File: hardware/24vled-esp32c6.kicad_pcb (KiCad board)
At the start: 2 copper layers, 26.4 x 90.8 mm, 20 parts, among them J1 2601-1106, J3 Barrel_Jack, Q1 AO3400A, Q2 AO3400A, Q3 AO3400A, Q4 AO3400A, Q5 AO3400A, U1 R-78E5.0-1.0

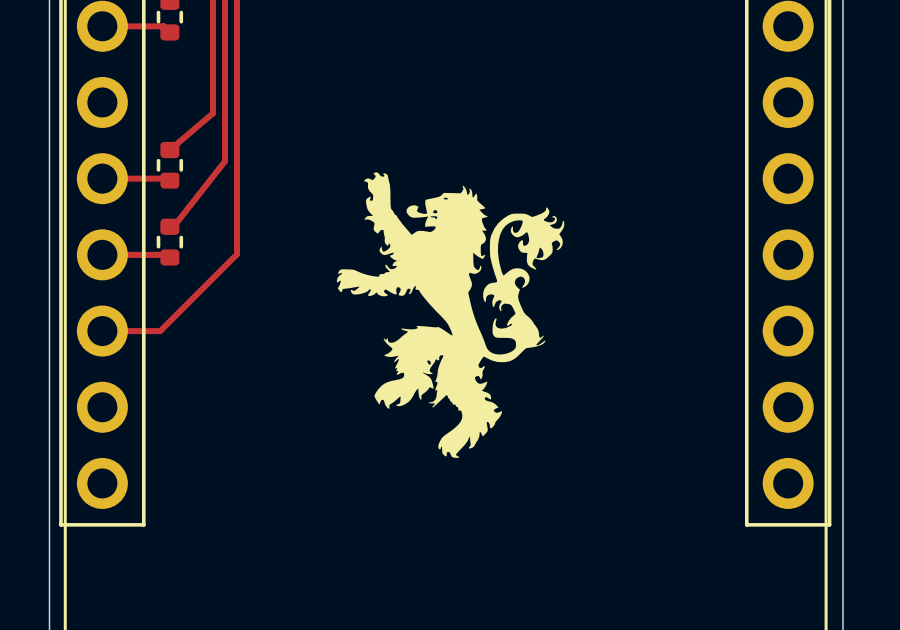
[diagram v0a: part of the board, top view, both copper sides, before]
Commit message: update pages
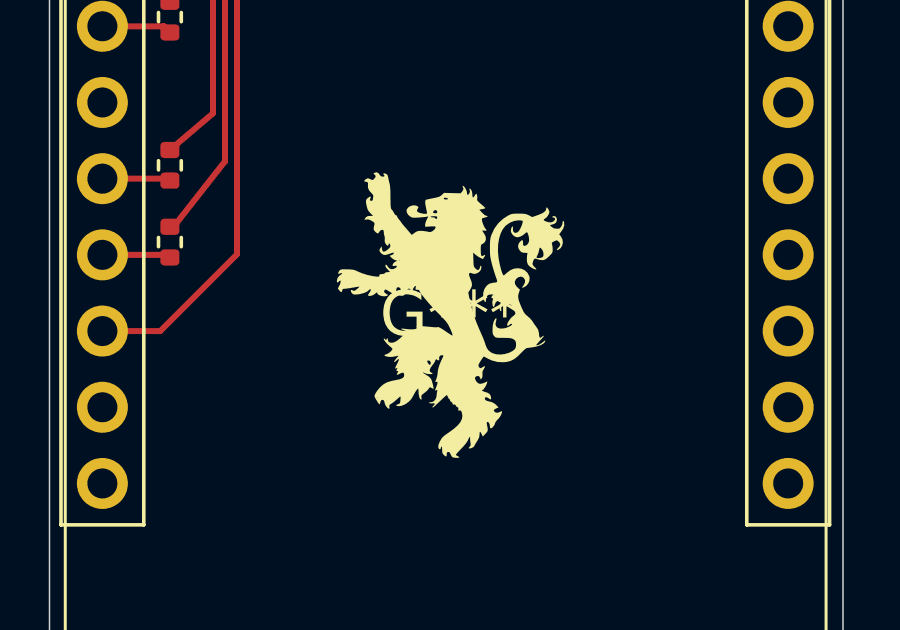
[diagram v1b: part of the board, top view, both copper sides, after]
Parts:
- G***: footprint Library:industries_10mm -> Internal:industries_10mm
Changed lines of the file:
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@@
 		)
 	)
-	(footprint "Library:industries_10mm"
+	(footprint "Internal:industries_10mm"
 		(layer "F.Cu")
 		(at 151.1 112.5)
@@
 			(at 0 0 0)
 			(layer "F.SilkS")
-			(hide yes)
 			(effects
 				(font
